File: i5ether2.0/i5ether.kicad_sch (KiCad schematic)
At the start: 6 parts, among them P1 Conn_02x15_Counter_Clockwise, P2 Conn_02x15_Counter_Clockwise, P3 Conn_02x15_Counter_Clockwise, P4 Conn_02x15_Counter_Clockwise, P5 Conn_02x15_Counter_Clockwise, P6 Conn_02x15_Counter_Clockwise

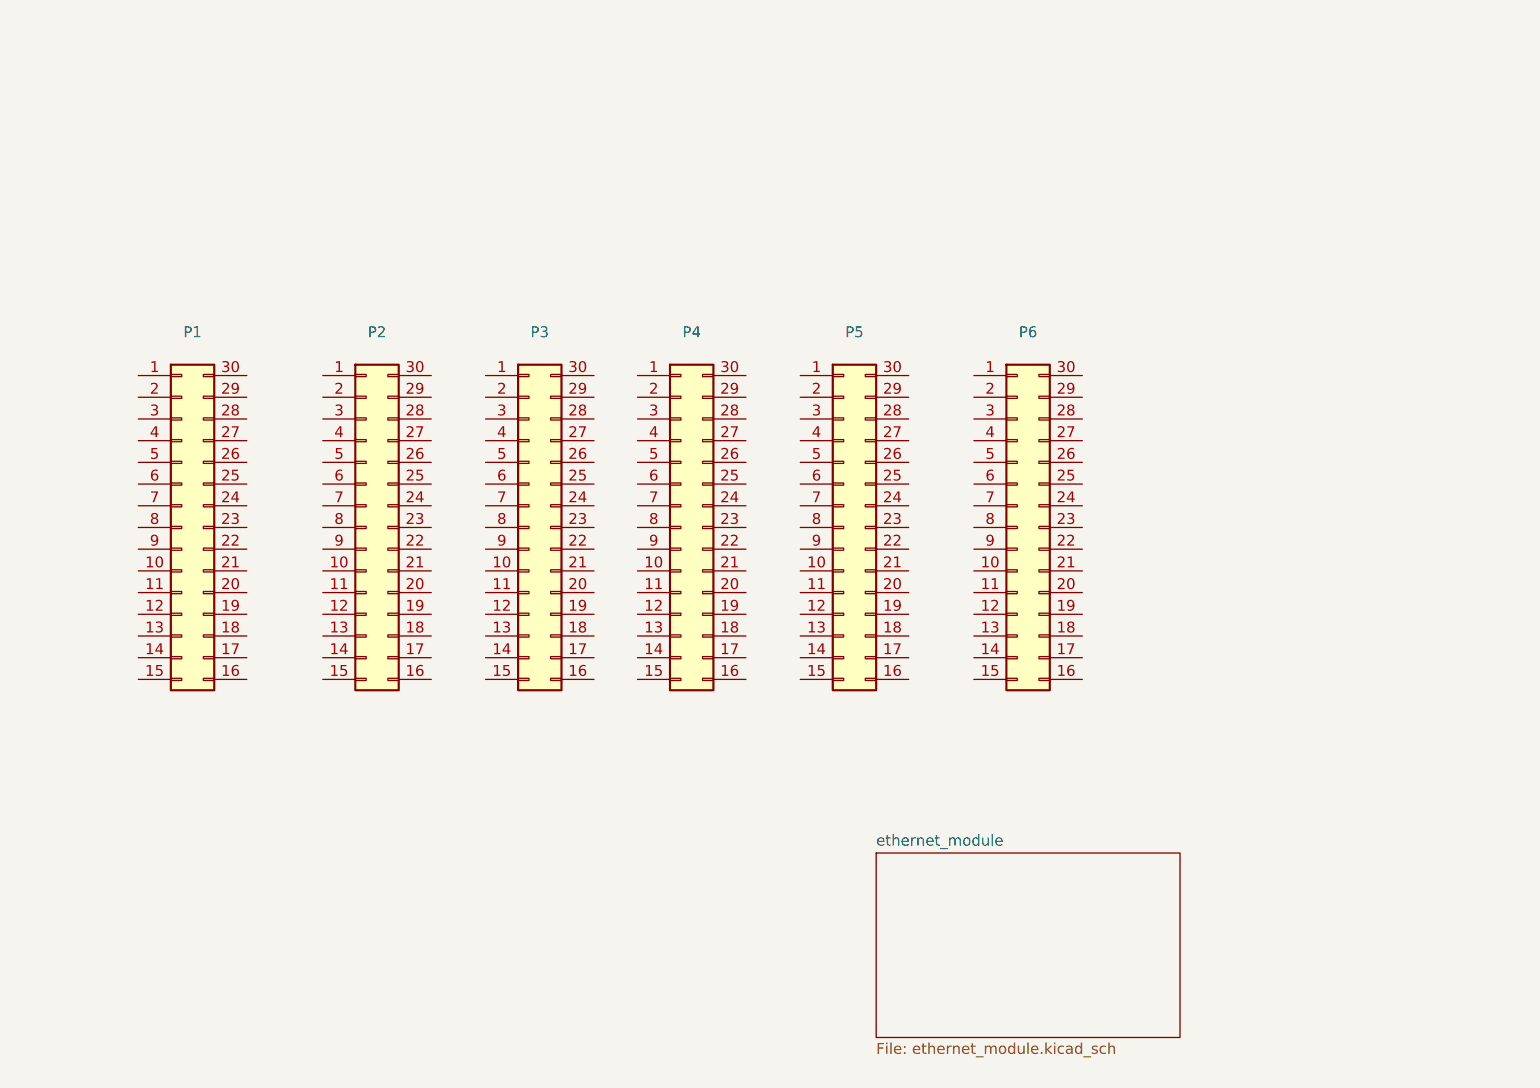
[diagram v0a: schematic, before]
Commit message: Essquematico con pantalla
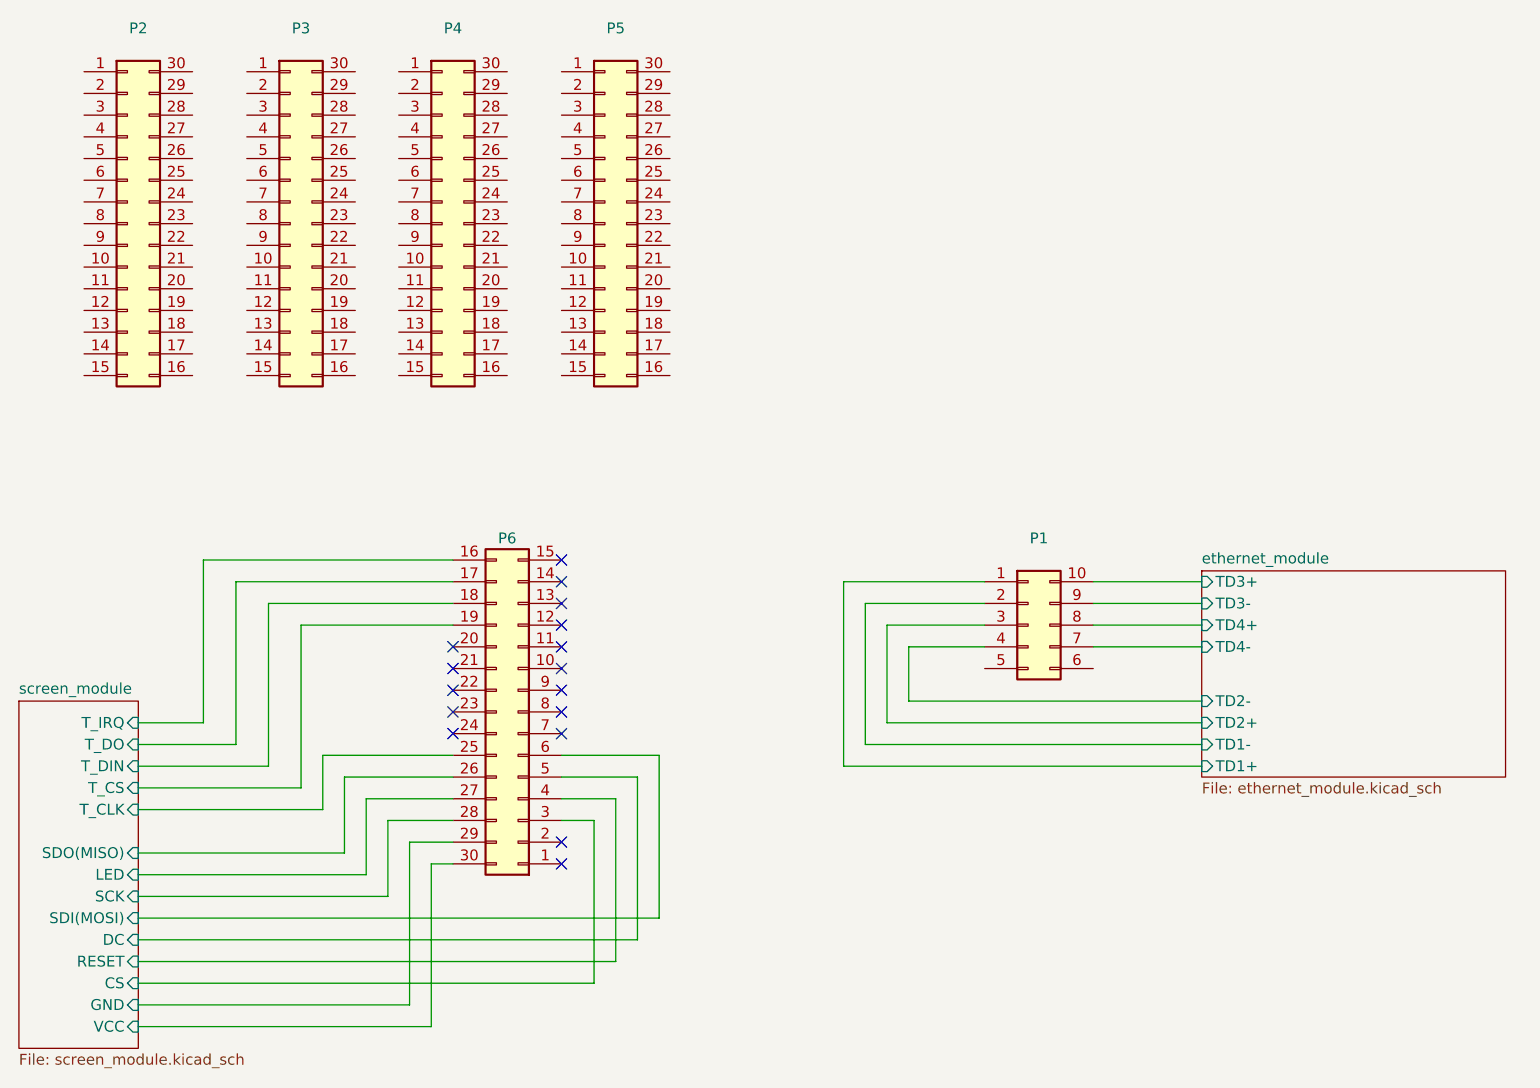
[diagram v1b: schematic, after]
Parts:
- removed P1: Conn_02x15_Counter_Clockwise, symbol Connector_Generic:Conn_02x15_Counter_Clockwise
- added P1: Conn_02x05_Counter_Clockwise, symbol Connector_Generic:Conn_02x05_Counter_Clockwise
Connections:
- net screen_module/T_IRQ: now reaches P6.16 (Pin_16)
- net screen_module/T_DO: now reaches P6.17 (Pin_17)
- net screen_module/T_DIN: now reaches P6.18 (Pin_18)
- net screen_module/T_CS: now reaches P6.19 (Pin_19)
- net screen_module/T_CLK: now reaches P6.25 (Pin_25)
- net screen_module/SDO(MISO): now reaches P6.26 (Pin_26)
- net screen_module/LED: now reaches P6.27 (Pin_27)
- net screen_module/SCK: now reaches P6.28 (Pin_28)
- net screen_module/GND: now reaches P6.29 (Pin_29)
- net screen_module/CS: now reaches P6.3 (Pin_3)
- net screen_module/VCC: now reaches P6.30 (Pin_30)
- net screen_module/RESET: now reaches P6.4 (Pin_4)
- net screen_module/DC: now reaches P6.5 (Pin_5)
- net screen_module/SDI(MOSI): now reaches P6.6 (Pin_6)
- new net ethernet_module/TD1+: P1.1 (Pin_1)
- new net ethernet_module/TD1-: P1.2 (Pin_2)
- new net ethernet_module/TD2+: P1.3 (Pin_3)
- new net ethernet_module/TD2-: P1.4 (Pin_4)
- new net ethernet_module/TD3+: P1.10 (Pin_10)
- new net ethernet_module/TD3-: P1.9 (Pin_9)
- new net ethernet_module/TD4+: P1.8 (Pin_8)
- new net ethernet_module/TD4-: P1.7 (Pin_7)
- no-connect marks 0 -> 16
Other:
- added sheet screen_module (screen_module.kicad_sch)
- sheet ethernet_module ports: added TD1+, TD1-, TD2+, TD2-, TD3+, TD3-, TD4+, TD4-; removed none
- moved on the sheet: P2, P3, P4, P5
